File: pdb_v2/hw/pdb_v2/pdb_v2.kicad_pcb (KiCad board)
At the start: 4 copper layers, 86.4 x 73.3 mm, 75 parts, among them J1 XT30-M_Ver, J2 JST-PH_01x02, J3 Conn_01x06_Pin, J5 JST-PH_01x02, J6 Conn_01x03, J7 Conn_01x03, J8 Conn_01x04, Q1 60Vds, SW1 SW_Push, SW2 SW_Push, U1 LMR51635XFDDCR, U2 ESP32-WROOM-32, U3 AP63203WU-7

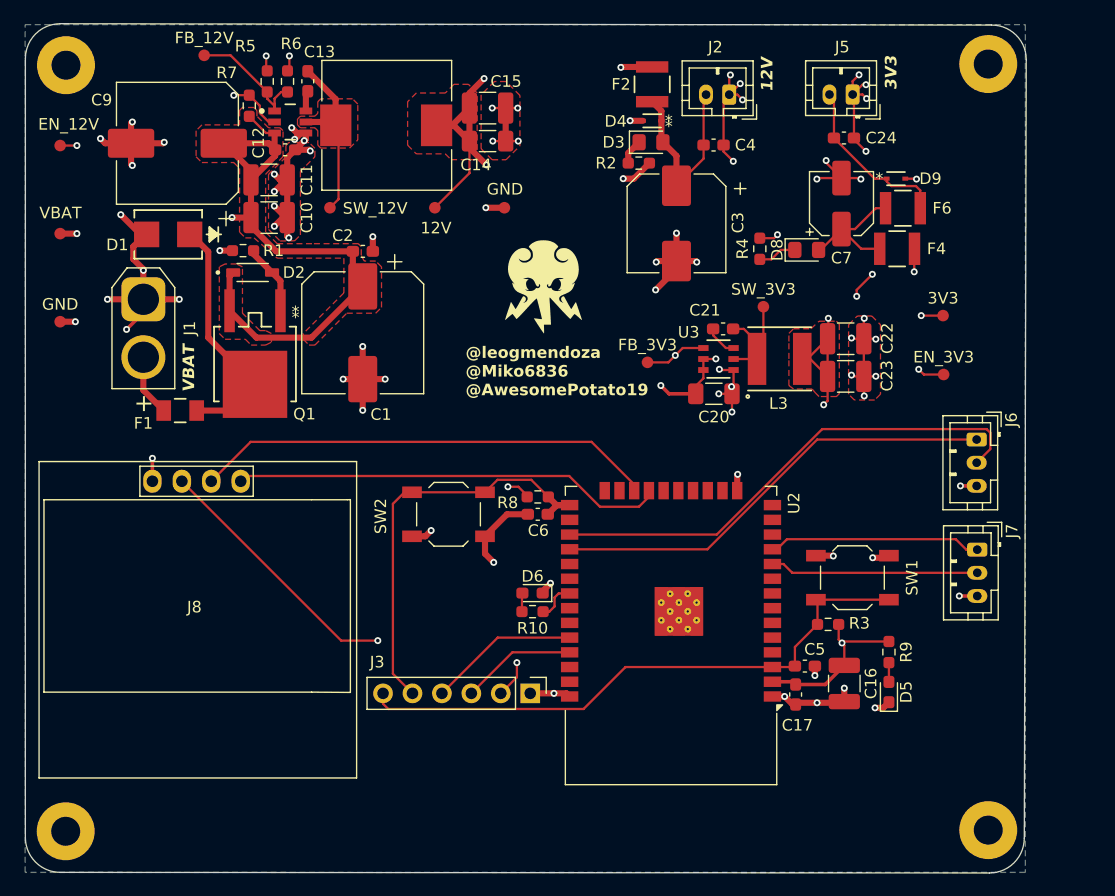
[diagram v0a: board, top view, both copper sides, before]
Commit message: Layout Update
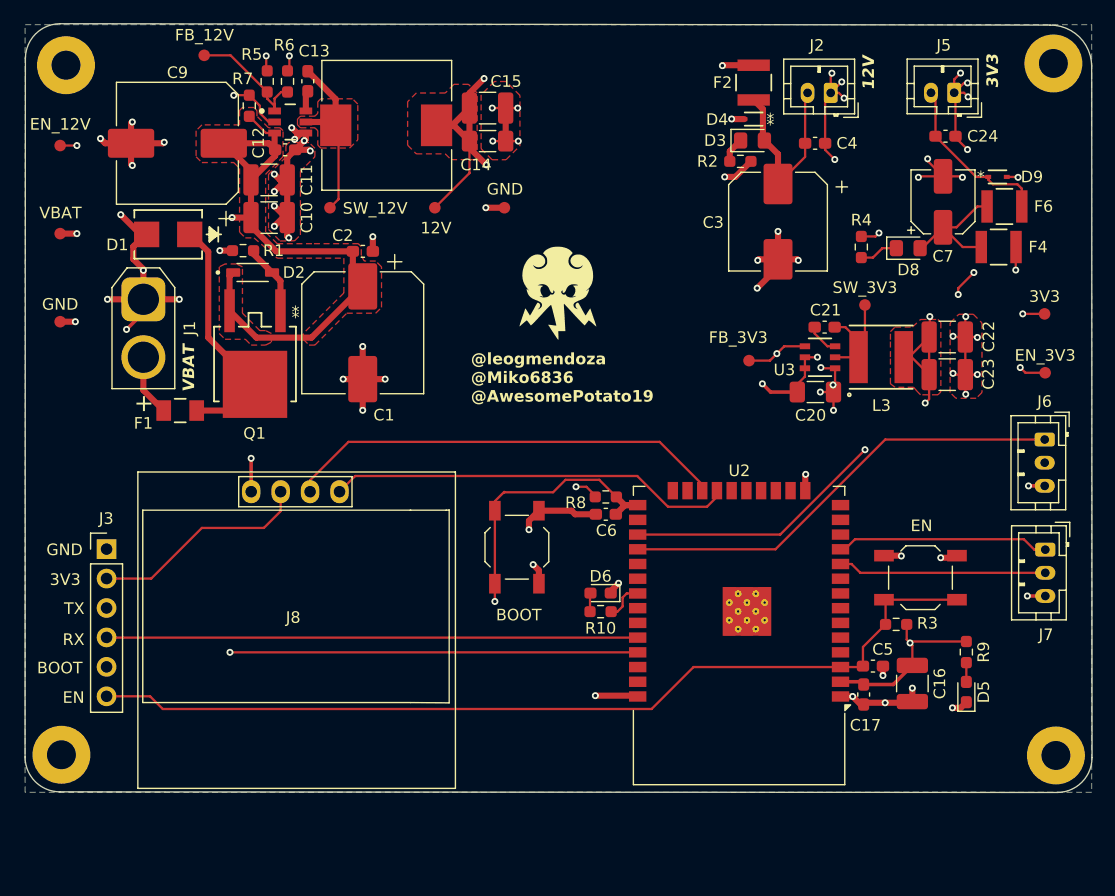
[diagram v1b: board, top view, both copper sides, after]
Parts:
- moved J3 38.6 mm to (19.0, 57.4), turned to 0 degrees
- moved C20 8.76 mm to (80.2, 43.8)
- moved C21 8.76 mm to (81.0, 38.2)
- moved C22 8.76 mm to (91.6, 39.1)
- moved C23 8.76 mm to (91.6, 42.3)
- moved C7 8.76 mm to (91.2, 27.4)
- moved D3 8.76 mm to (74.8, 22.1)
- moved D4 8.76 mm to (74.9, 20.2)
- moved D8 8.76 mm to (88.2, 31.4)
- moved EN_3V3 8.76 mm to (100.0, 42.1)
- moved F2 8.76 mm to (74.9, 17.1)
- moved F4 8.76 mm to (96.0, 31.3)
- moved F6 8.76 mm to (96.5, 27.8)
- moved J2 8.76 mm to (81.5, 18.0)
- moved L3 8.76 mm to (85.9, 40.8)
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- renumbered SW2 to BOOT, SW1 to EN
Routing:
- net /TX: track 9.95 -> 47.5 mm, vias 0 -> 1
- net /RX: track 13.0 -> 45.8 mm
- net /EN: track 51.1 -> 80.1 mm
- net /BOOT: track 36.3 -> 60.7 mm, vias 0 -> 1
- net 12V_BUS: track 131.2 -> 148.3 mm
- net /BMS RX: track 43.3 -> 38.6 mm, vias 0 -> 1
- net /OLED SDA: track 37.4 -> 35.1 mm
- net /OLED SCL: track 40.0 -> 38.3 mm
- net 3V3_BUS: track 167.6 -> 166.2 mm, vias 11 -> 9
- net GND: track 166.6 -> 167.4 mm
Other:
- board size 86.4 x 73.3 mm -> 92.1 x 66.3 mm
- board text added: "BOOT"
- board text added: "EN"
- board text added: "GND"
- board text added: "RX"
- board text added: "TX"
